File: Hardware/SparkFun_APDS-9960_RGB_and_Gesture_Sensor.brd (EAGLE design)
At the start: 15.2 x 20.3 mm, 19 parts, among them U1 APDS-9960

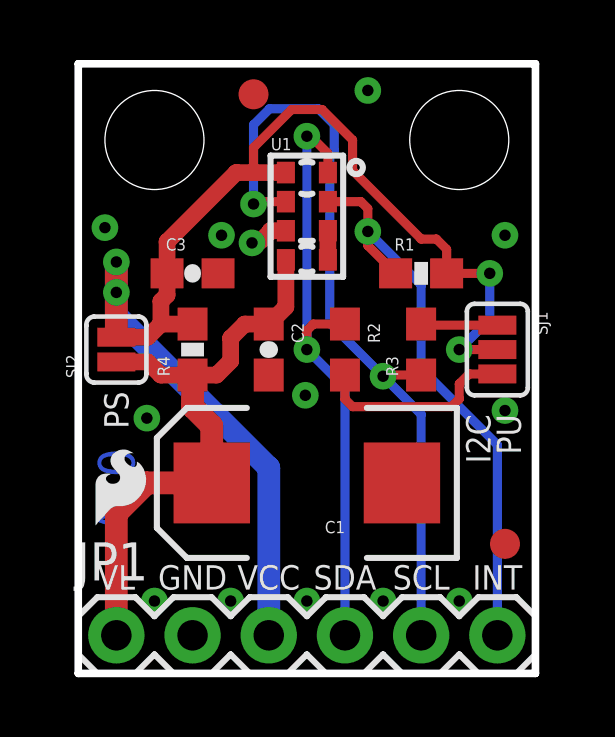
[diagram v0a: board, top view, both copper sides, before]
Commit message: Changed 4.7k resistors to proper 0603-RES package.
This adds a small silkscreen dot under the resistor.
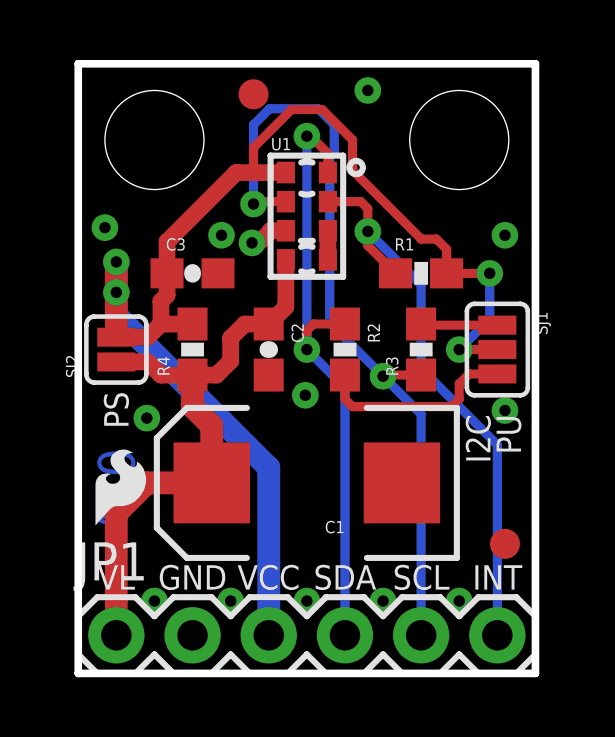
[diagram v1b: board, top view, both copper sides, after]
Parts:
- R2, R3: value 4.7k -> 4.7K; device SparkFun-Resistors:0603 -> SparkFun-Resistors:0603-RES
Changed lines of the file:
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@@
 <?xml version="1.0" encoding="utf-8"?>
 <!DOCTYPE eagle SYSTEM "eagle.dtd">
-<eagle version="6.5.0">
+<eagle version="7.2.0">
 <drawing>
 <settings>
@@
 <pass name="Default">
 <param name="RoutingGrid" value="50mil"/>
+<param name="AutoGrid" value="1"/>
+<param name="Efforts" value="0"/>
+<param name="TopRouterVariant" value="1"/>
 <param name="tpViaShape" value="round"/>
 <param name="PrefDir.1" value="|"/>
@@
 <attribute name="VALUE" value="10K" x="11.43" y="13.335" size="1.778" layer="27" display="off"/>
 </element>
-<element name="R2" library="SparkFun-Resistors" package="0603" value="4.7k" x="8.89" y="10.795" rot="R270">
+<element name="R2" library="SparkFun-Resistors" package="0603-RES" value="4.7K" x="8.89" y="10.795" rot="R270">
 <attribute name="PROD_ID" value="RES-07857" x="-15.24" y="-8.255" size="1.778" layer="27" rot="R270" display="off"/>
+<attribute name="VALUE" value="4.7K" x="8.89" y="10.795" size="1.778" layer="27" rot="R270" display="off"/>
 </element>
 <element name="SJ1" library="SparkFun-Passives" package="SJ_3_PASTE1&amp;2&amp;3" value="" x="13.97" y="10.795" rot="R270"/>
@@
 <element name="LOGO2" library="SparkFun-Aesthetics" package="OSHW-LOGO-S" value="OSHW-LOGOS" x="7.62" y="17.78" rot="MR0"/>
 <element name="R4" library="SparkFun-Resistors" package="0603-RES" value="DNP" x="3.81" y="10.795" rot="R90"/>
-<element name="R3" library="SparkFun-Resistors" package="0603" value="4.7k" x="11.43" y="10.795" rot="R90">
+<element name="R3" library="SparkFun-Resistors" package="0603-RES" value="4.7K" x="11.43" y="10.795" rot="R90">
 <attribute name="PROD_ID" value="RES-07857" x="11.43" y="10.795" size="1.778" layer="27" font="vector" ratio="15" rot="R90" display="off"/>
+<attribute name="VALUE" value="4.7K" x="11.43" y="10.795" size="1.778" layer="27" rot="R90" display="off"/>
 </element>
 <element name="SJ2" library="SparkFun-Retired" package="SJ_2S" value="SOLDERJUMPERNC" x="1.27" y="10.795" rot="R90"/>

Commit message: Reverting to current board layout files
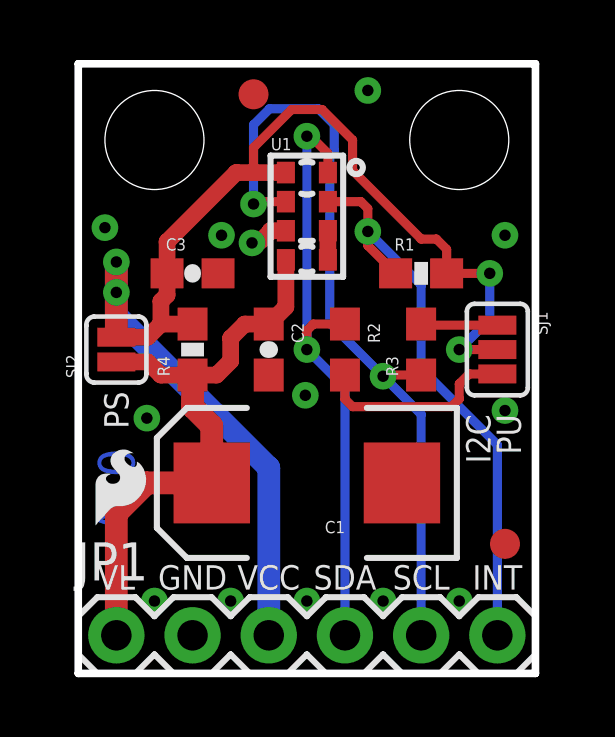
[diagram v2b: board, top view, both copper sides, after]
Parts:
- R2, R3: value 4.7K -> 4.7k; device SparkFun-Resistors:0603-RES -> SparkFun-Resistors:0603
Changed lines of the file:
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@@
 <?xml version="1.0" encoding="utf-8"?>
 <!DOCTYPE eagle SYSTEM "eagle.dtd">
-<eagle version="7.2.0">
+<eagle version="6.5.0">
 <drawing>
 <settings>
@@
 <pass name="Default">
 <param name="RoutingGrid" value="50mil"/>
-<param name="AutoGrid" value="1"/>
-<param name="Efforts" value="0"/>
-<param name="TopRouterVariant" value="1"/>
 <param name="tpViaShape" value="round"/>
 <param name="PrefDir.1" value="|"/>
@@
 <attribute name="VALUE" value="10K" x="11.43" y="13.335" size="1.778" layer="27" display="off"/>
 </element>
-<element name="R2" library="SparkFun-Resistors" package="0603-RES" value="4.7K" x="8.89" y="10.795" rot="R270">
+<element name="R2" library="SparkFun-Resistors" package="0603" value="4.7k" x="8.89" y="10.795" rot="R270">
 <attribute name="PROD_ID" value="RES-07857" x="-15.24" y="-8.255" size="1.778" layer="27" rot="R270" display="off"/>
-<attribute name="VALUE" value="4.7K" x="8.89" y="10.795" size="1.778" layer="27" rot="R270" display="off"/>
 </element>
 <element name="SJ1" library="SparkFun-Passives" package="SJ_3_PASTE1&amp;2&amp;3" value="" x="13.97" y="10.795" rot="R270"/>
@@
 <element name="LOGO2" library="SparkFun-Aesthetics" package="OSHW-LOGO-S" value="OSHW-LOGOS" x="7.62" y="17.78" rot="MR0"/>
 <element name="R4" library="SparkFun-Resistors" package="0603-RES" value="DNP" x="3.81" y="10.795" rot="R90"/>
-<element name="R3" library="SparkFun-Resistors" package="0603-RES" value="4.7K" x="11.43" y="10.795" rot="R90">
+<element name="R3" library="SparkFun-Resistors" package="0603" value="4.7k" x="11.43" y="10.795" rot="R90">
 <attribute name="PROD_ID" value="RES-07857" x="11.43" y="10.795" size="1.778" layer="27" font="vector" ratio="15" rot="R90" display="off"/>
-<attribute name="VALUE" value="4.7K" x="11.43" y="10.795" size="1.778" layer="27" rot="R90" display="off"/>
 </element>
 <element name="SJ2" library="SparkFun-Retired" package="SJ_2S" value="SOLDERJUMPERNC" x="1.27" y="10.795" rot="R90"/>
